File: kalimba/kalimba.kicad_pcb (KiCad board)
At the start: 2 copper layers, 174 x 101.9 mm, 25 parts, among them J2 Conn_01x08, J3 Conn_01x08, SW1 SW_SPDT, U1 WS2812B-2020, U10 WS2812B-2020, U11 WS2812B-2020, U12 WS2812B-2020, U13 WS2812B-2020, U14 WS2812B-2020, U15 WS2812B-2020, U16 WS2812B-2020, U17 WS2812B-2020, U18 WS2812B-2020, U19 WS2812B-2020, U2 WS2812B-2020, U20 WS2812B-2020, U21 WS2812B-2020, U3 WS2812B-2020, U4 WS2812B-2020, U5 WS2812B-2020, U6 WS2812B-2020, U7 WS2812B-2020, U8 WS2812B-2020, U9 WS2812B-2020

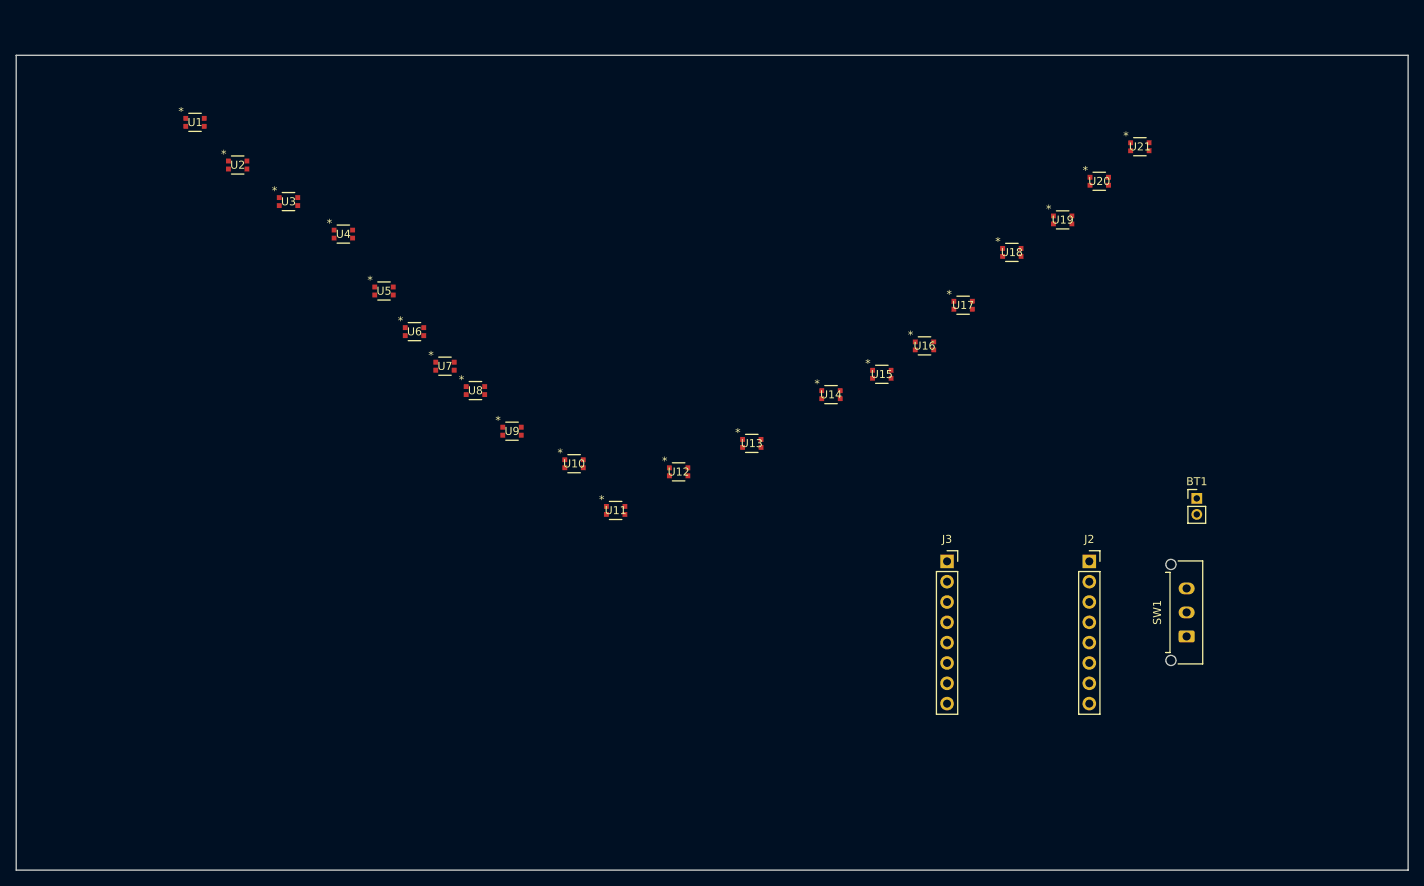
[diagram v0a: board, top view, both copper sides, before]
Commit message: hey
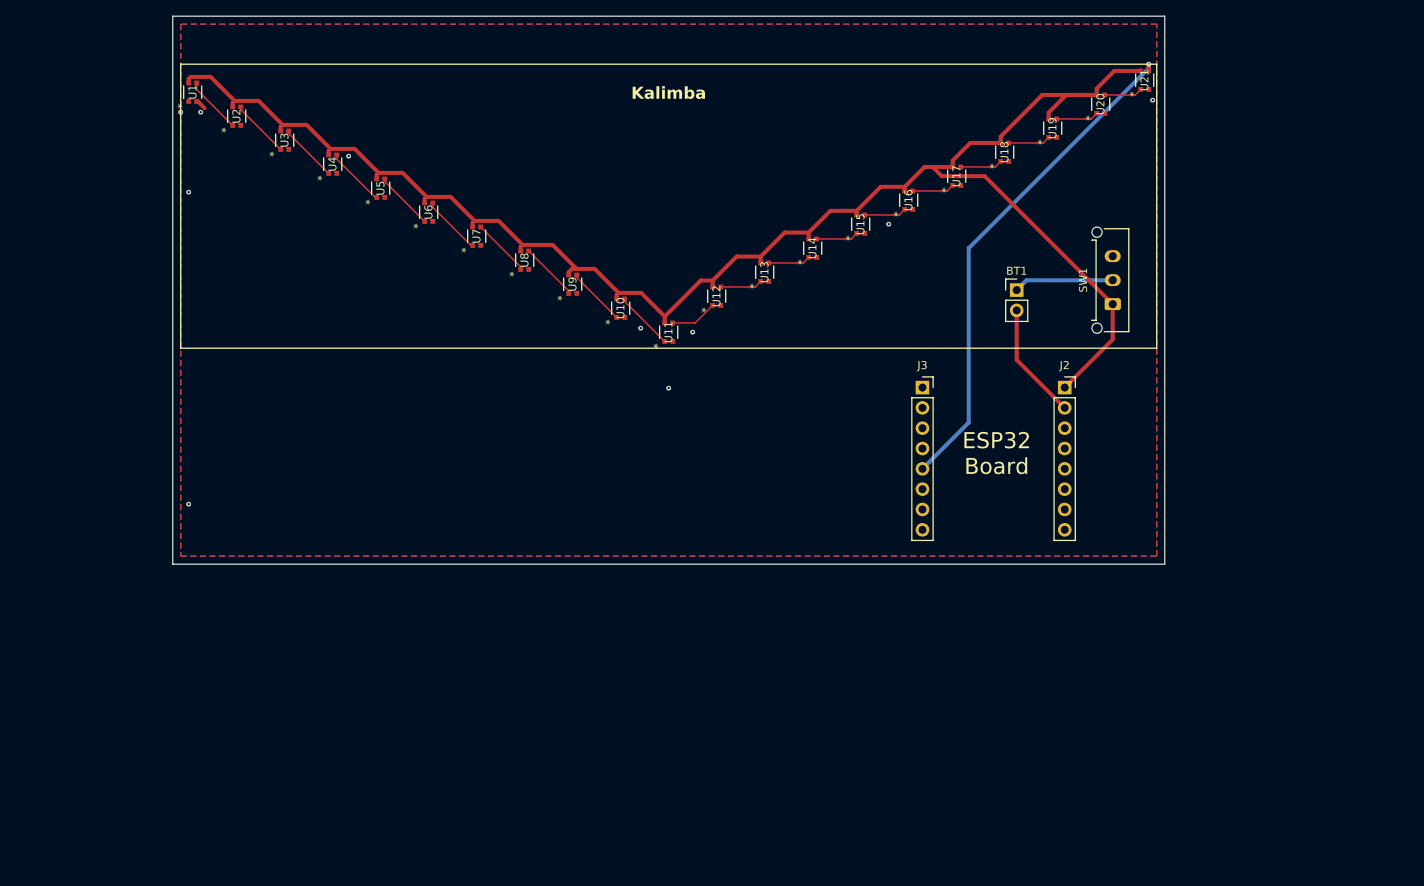
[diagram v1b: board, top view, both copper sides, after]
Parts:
- BT1: footprint Connector_PinHeader_2.00mm:PinHeader_1x02_P2.00mm_Vertical -> Connector_PinHeader_2.54mm:PinHeader_1x02_P2.54mm_Vertical
- moved SW1 42.5 mm to (196.5, 71.5)
- moved BT1 34.4 mm to (184.5, 69.7)
- moved U11 23.2 mm to (141.0, 75.0), turned to 90 degrees
- moved U12 22.5 mm to (147.0, 70.5), turned to 90 degrees
- moved J2 21.9 mm to (190.5, 81.9)
- moved J3 21.9 mm to (172.7, 81.9)
- moved U13 21.5 mm to (153.0, 67.5), turned to 90 degrees
- moved U10 20.3 mm to (135.0, 72.0), turned to 90 degrees
- moved U9 19.9 mm to (129.0, 69.0), turned to 90 degrees
- moved U15 18.9 mm to (165.0, 61.5), turned to 90 degrees
- moved U14 18.4 mm to (159.0, 64.5), turned to 90 degrees
- moved U16 18.3 mm to (171.0, 58.5), turned to 90 degrees
- moved U8 17.4 mm to (123.0, 66.0), turned to 90 degrees
- moved U7 16.7 mm to (117.0, 63.0), turned to 90 degrees
- moved U17 16.1 mm to (177.0, 55.5), turned to 90 degrees
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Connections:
- U1 pad 1: Net-(J3-Pin_5) -> unconnected-(U1-DO-Pad1)
- U21 pad 3: unconnected-(U21-DI-Pad3) -> Net-(J3-Pin_5)
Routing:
- net +5V: track 0.00 -> 209.0 mm
- net Net-(J3-Pin_5): track 0.00 -> 63.1 mm, vias 0 -> 1
- net GND: track 0.00 -> 16.3 mm, vias 0 -> 10
- net Net-(BT1-+): track 0.00 -> 12.5 mm
- net Net-(U6-DI): track 0.00 -> 7.51 mm
- net Net-(U4-DI): track 0.00 -> 7.50 mm
- net Net-(U5-DI): track 0.00 -> 7.38 mm
- net Net-(U3-DI): track 0.00 -> 7.38 mm
- net Net-(U2-DI): track 0.00 -> 7.38 mm
- net Net-(U7-DI): track 0.00 -> 7.38 mm
- net Net-(U8-DI): track 0.00 -> 7.38 mm
- net Net-(U10-DO): track 0.00 -> 7.38 mm
- net Net-(U10-DI): track 0.00 -> 7.38 mm
- net Net-(U1-DI): track 0.00 -> 7.18 mm
- net Net-(U11-DI): track 0.00 -> 5.91 mm
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- added copper zone on B.Cu, net GND
- added copper zone on F.Cu, net GND
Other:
- board size 174 x 101.9 mm -> 124 x 68.5 mm
- board text added: "ESP32 Board"
- board text added: "Kalimba"
